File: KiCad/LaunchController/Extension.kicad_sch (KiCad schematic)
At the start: 3 parts, among them J17 CONN_STATUS_PANEL, J22 CONN_PANEL_BAORD_2, J23 CONN_PANEL_BAORD_1

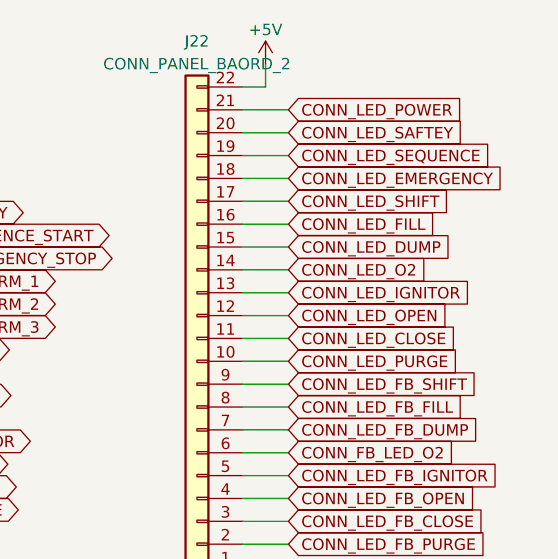
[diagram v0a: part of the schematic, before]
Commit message: 配線終わらん
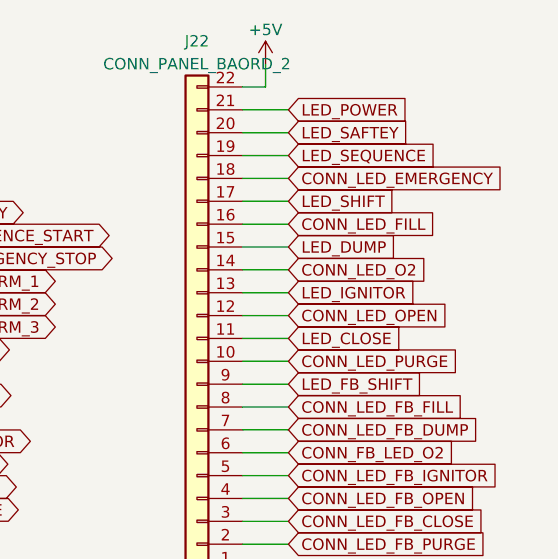
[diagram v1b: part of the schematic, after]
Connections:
- net CONN_LED_CLOSE renamed LED_CLOSE
- net CONN_LED_DUMP renamed LED_DUMP
- net CONN_LED_FB_SHIFT renamed LED_FB_SHIFT
- net CONN_LED_IGNITOR renamed LED_IGNITOR
- net CONN_LED_POWER renamed LED_POWER
- net CONN_LED_SAFTEY renamed LED_SAFTEY
- net CONN_LED_SEQUENCE renamed LED_SEQUENCE
- net CONN_LED_SHIFT renamed LED_SHIFT
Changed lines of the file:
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@@
     )
   )
-  (global_label "CONN_LED_SEQUENCE" (shape input) (at 130.81 40.64 0) (fields_autoplaced)
+  (global_label "LED_SEQUENCE" (shape input) (at 130.81 40.64 0) (fields_autoplaced)
     (effects (font (size 1.27 1.27)) (justify left))
-    (property "Intersheetrefs" "${INTERSHEET_REFS}" (at 154.2776 40.64 0)
+    (property "Intersheetrefs" "${INTERSHEET_REFS}" (at 148.0485 40.64 0)
       (effects (font (size 1.27 1.27)) (justify left) hide)
     )
   )
-  (global_label "CONN_LED_SAFTEY" (shape input) (at 130.81 38.1 0) (fields_autoplaced)
+  (global_label "LED_SAFTEY" (shape input) (at 130.81 38.1 0) (fields_autoplaced)
     (effects (font (size 1.27 1.27)) (justify left))
-    (property "Intersheetrefs" "${INTERSHEET_REFS}" (at 150.9515 38.1 0)
+    (property "Intersheetrefs" "${INTERSHEET_REFS}" (at 144.7224 38.1 0)
       (effects (font (size 1.27 1.27)) (justify left) hide)
     )
@@
     )
   )
-  (global_label "CONN_LED_FB_SHIFT" (shape input) (at 130.81 66.04 0) (fields_autoplaced)
+  (global_label "LED_FB_SHIFT" (shape input) (at 130.81 66.04 0) (fields_autoplaced)
     (effects (font (size 1.27 1.27)) (justify left))
-    (property "Intersheetrefs" "${INTERSHEET_REFS}" (at 152.8868 66.04 0)
+    (property "Intersheetrefs" "${INTERSHEET_REFS}" (at 146.6577 66.04 0)
       (effects (font (size 1.27 1.27)) (justify left) hide)
     )
@@
     )
   )
-  (global_label "CONN_LED_POWER" (shape input) (at 130.81 35.56 0) (fields_autoplaced)
+  (global_label "LED_POWER" (shape input) (at 130.81 35.56 0) (fields_autoplaced)
     (effects (font (size 1.27 1.27)) (justify left))
-    (property "Intersheetrefs" "${INTERSHEET_REFS}" (at 150.8305 35.56 0)
+    (property "Intersheetrefs" "${INTERSHEET_REFS}" (at 144.6014 35.56 0)
       (effects (font (size 1.27 1.27)) (justify left) hide)
     )
   )
-  (global_label "CONN_LED_IGNITOR" (shape input) (at 130.81 55.88 0) (fields_autoplaced)
+  (global_label "LED_IGNITOR" (shape input) (at 130.81 55.88 0) (fields_autoplaced)
     (effects (font (size 1.27 1.27)) (justify left))
-    (property "Intersheetrefs" "${INTERSHEET_REFS}" (at 151.7378 55.88 0)
+    (property "Intersheetrefs" "${INTERSHEET_REFS}" (at 145.5087 55.88 0)
       (effects (font (size 1.27 1.27)) (justify left) hide)
     )
@@
     )
   )
-  (global_label "CONN_LED_SHIFT" (shape input) (at 130.81 45.72 0) (fields_autoplaced)
+  (global_label "LED_SHIFT" (shape input) (at 130.81 45.72 0) (fields_autoplaced)
     (effects (font (size 1.27 1.27)) (justify left))
-    (property "Intersheetrefs" "${INTERSHEET_REFS}" (at 149.5606 45.72 0)
+    (property "Intersheetrefs" "${INTERSHEET_REFS}" (at 143.3315 45.72 0)
       (effects (font (size 1.27 1.27)) (justify left) hide)
     )
@@
     )
   )
-  (global_label "CONN_LED_DUMP" (shape input) (at 130.81 50.8 0) (fields_autoplaced)
+  (global_label "LED_DUMP" (shape input) (at 130.81 50.8 0) (fields_autoplaced)
     (effects (font (size 1.27 1.27)) (justify left))
-    (property "Intersheetrefs" "${INTERSHEET_REFS}" (at 149.6815 50.8 0)
+    (property "Intersheetrefs" "${INTERSHEET_REFS}" (at 143.4524 50.8 0)
       (effects (font (size 1.27 1.27)) (justify left) hide)
     )
@@
     )
   )
-  (global_label "CONN_LED_CLOSE" (shape input) (at 130.81 60.96 0) (fields_autoplaced)
+  (global_label "LED_CLOSE" (shape input) (at 130.81 60.96 0) (fields_autoplaced)
     (effects (font (size 1.27 1.27)) (justify left))
-    (property "Intersheetrefs" "${INTERSHEET_REFS}" (at 150.3467 60.96 0)
+    (property "Intersheetrefs" "${INTERSHEET_REFS}" (at 144.1176 60.96 0)
       (effects (font (size 1.27 1.27)) (justify left) hide)
     )
